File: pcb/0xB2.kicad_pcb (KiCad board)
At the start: 2 copper layers, 70.9 x 50.8 mm, 65 parts, among them J1 USB_C_Receptacle_USB2.0, J10 RGB, J11 serial, J12 Conn_01x02_Female, J13 Conn_01x02_Female, J14 Conn_01x02_Female, J15 Conn_01x02_Female, J5 Conn_01x02, J6 Ribbon, J7 Ribbon, J8 trackball, J9 Serial, SW2 SW_Push, SW3 SW_SPST, U1 RP2040, U2 GD25Q80CEIGR, U3 XC6210B332MR-G, Y1 Crystal_GND24

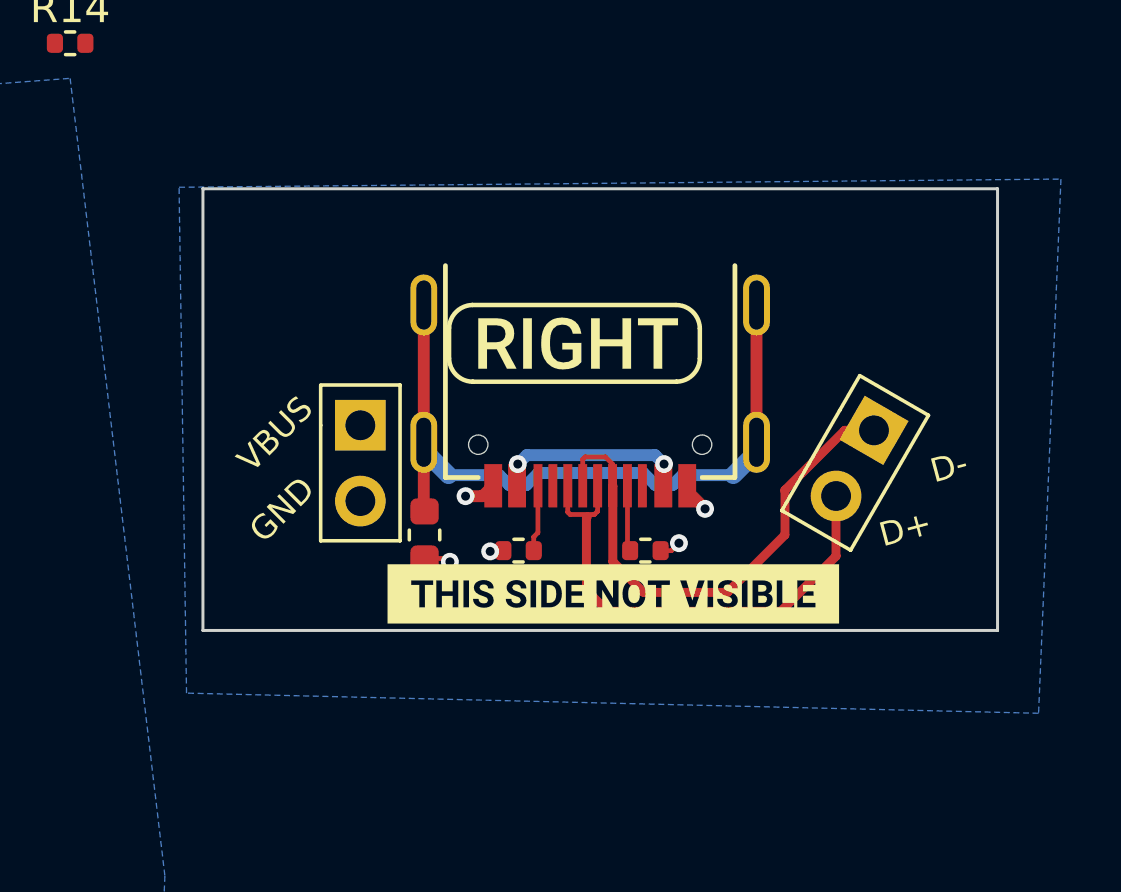
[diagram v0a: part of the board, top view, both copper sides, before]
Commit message: cleanup
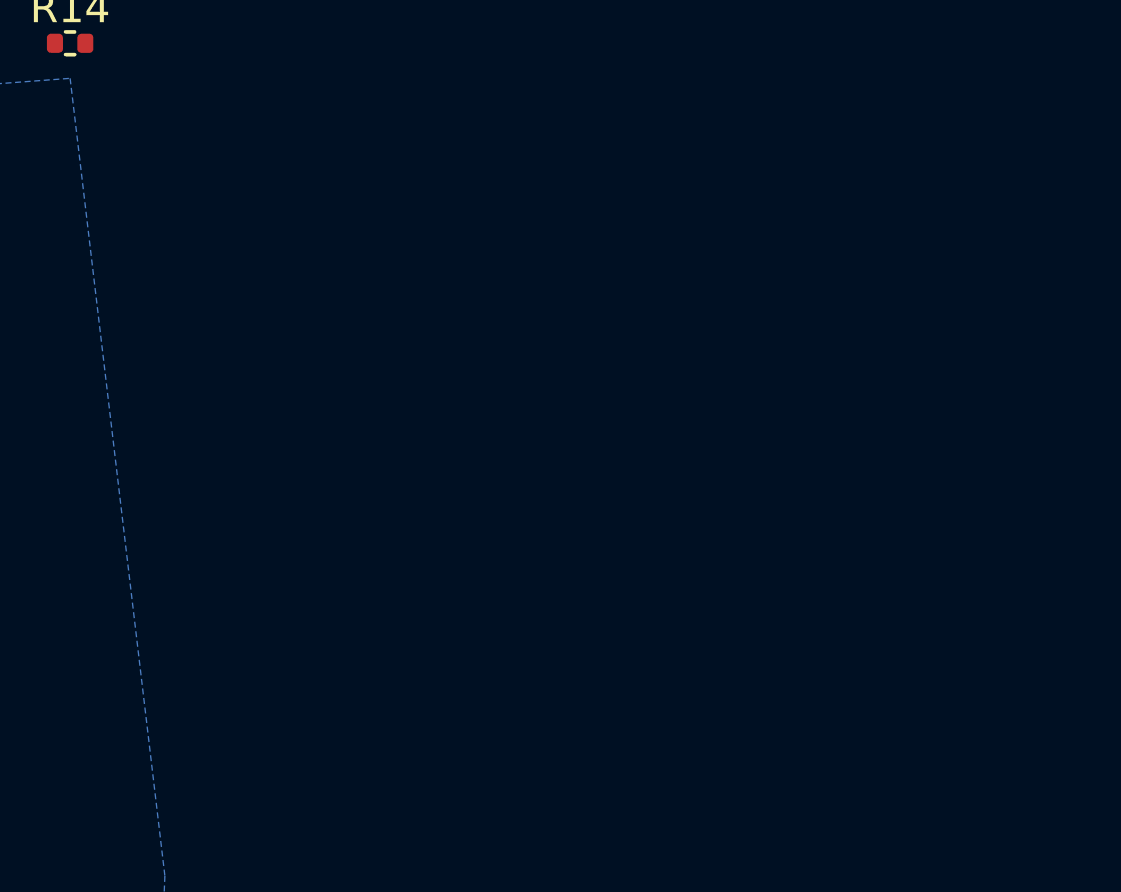
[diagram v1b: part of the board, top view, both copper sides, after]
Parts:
- removed FB1: FerriteBead_Small, Inductor_SMD:L_0603_1608Metric
- removed J1: USB_C_Receptacle_USB2.0, 0xLib_USB_Type-C:USB_C_Receptacle_HRO_TYPE-C-31-M-14
- removed J12, J13: Conn_01x02_Female, Library:PinHeader_1x02_P2.54mm_Vertical
- removed R4, R5: 5.1k, Resistor_SMD:R_0402_1005Metric
- removed kibuzzard-61F01B61 (x2): G***, kibuzzard-61F01B61
- removed kibuzzard-6284F97C: G***, kibuzzard-6284F97C
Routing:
- net Net-(FB1-Pad2): track 23.9 -> 0.00 mm
- net Net-(J1-PadA7): track 17.6 -> 0.00 mm
- net Net-(J1-PadA6): track 16.7 -> 0.00 mm
- net Net-(J1-PadA4): track 5.15 -> 0.00 mm, vias 2 -> 0
- net GND: track 42.0 -> 37.8 mm, vias 31 -> 26
- net Net-(J1-PadB5): track 2.23 -> 0.00 mm
- net Net-(J1-PadA5): track 2.21 -> 0.00 mm
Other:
- board size 70.9 x 50.8 mm -> 41.8 x 50.8 mm
- board text removed: "Solder on this side"
